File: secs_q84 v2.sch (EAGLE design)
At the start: 107 parts, among them IC1 MAX203ECWP, IC2 REF3440TIDBVR, IC3 ADP151AUJZ-3.3-R7, IC4 PIC18F47Q84-I_PT, IC5 MCZ33996EK, IC6 74HC125D, IC7 TIC12400DCPR

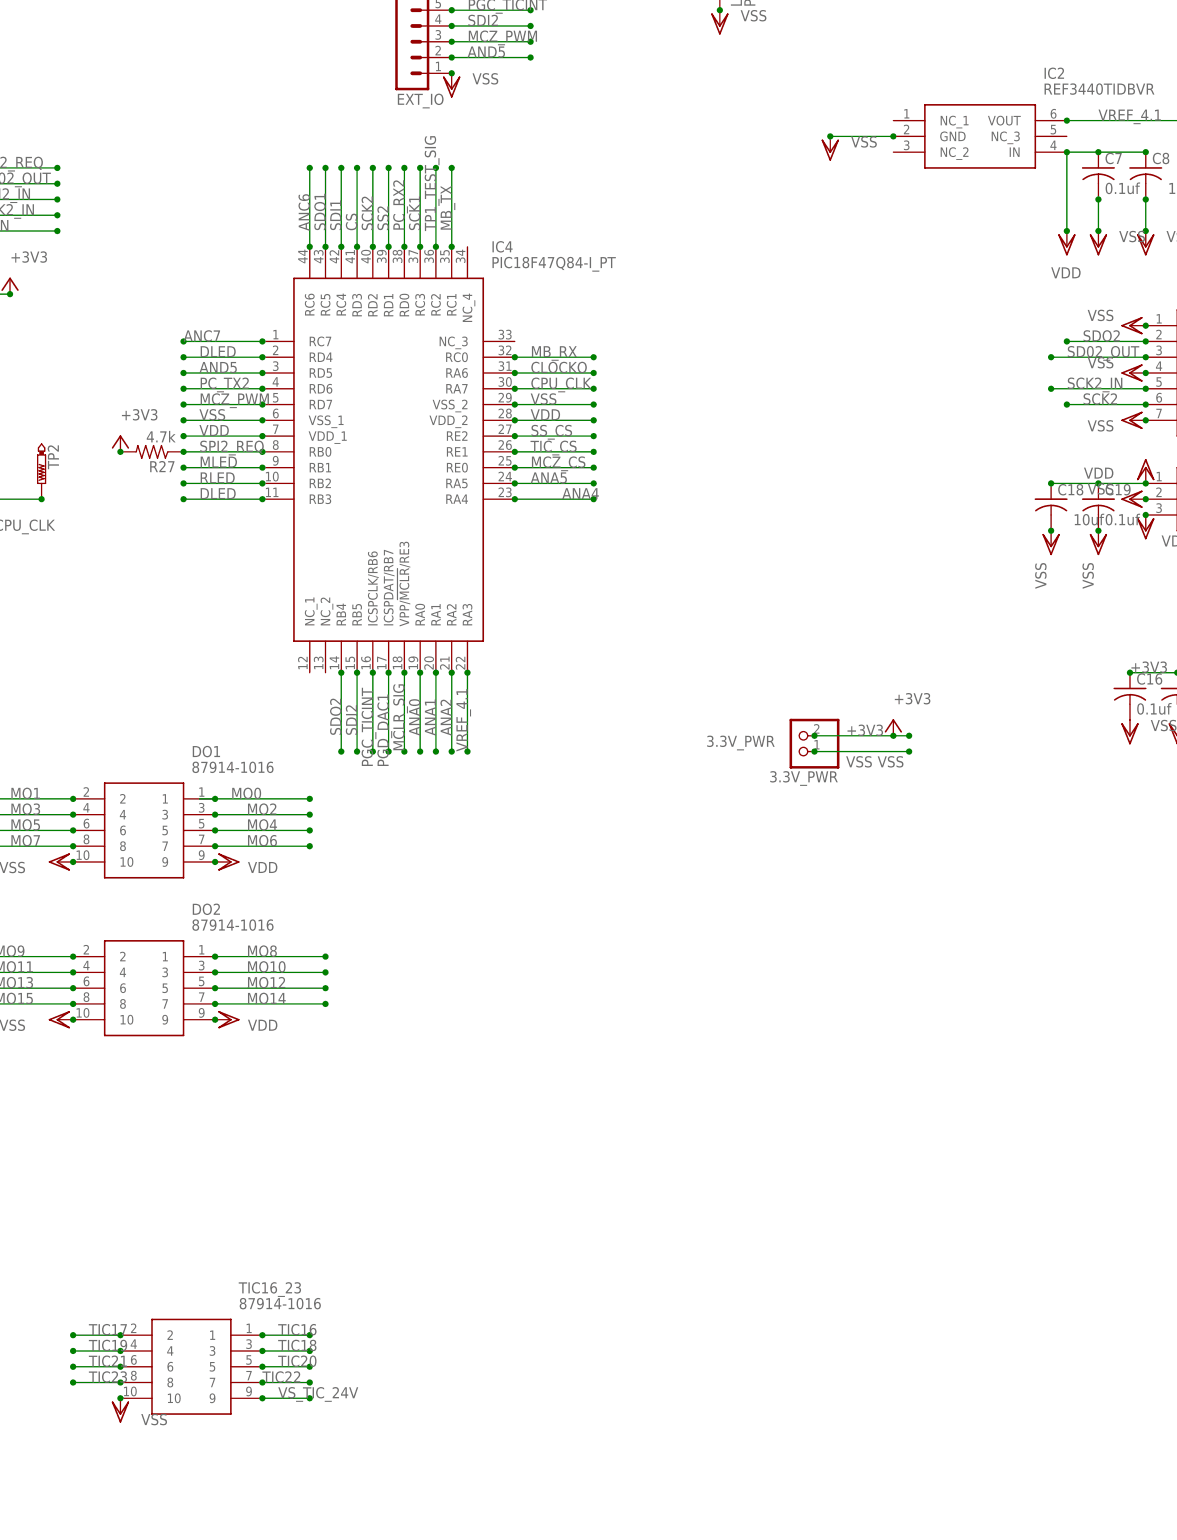
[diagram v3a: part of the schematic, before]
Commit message: up uuuppp#	modified:   secs_q84 v2.b#5
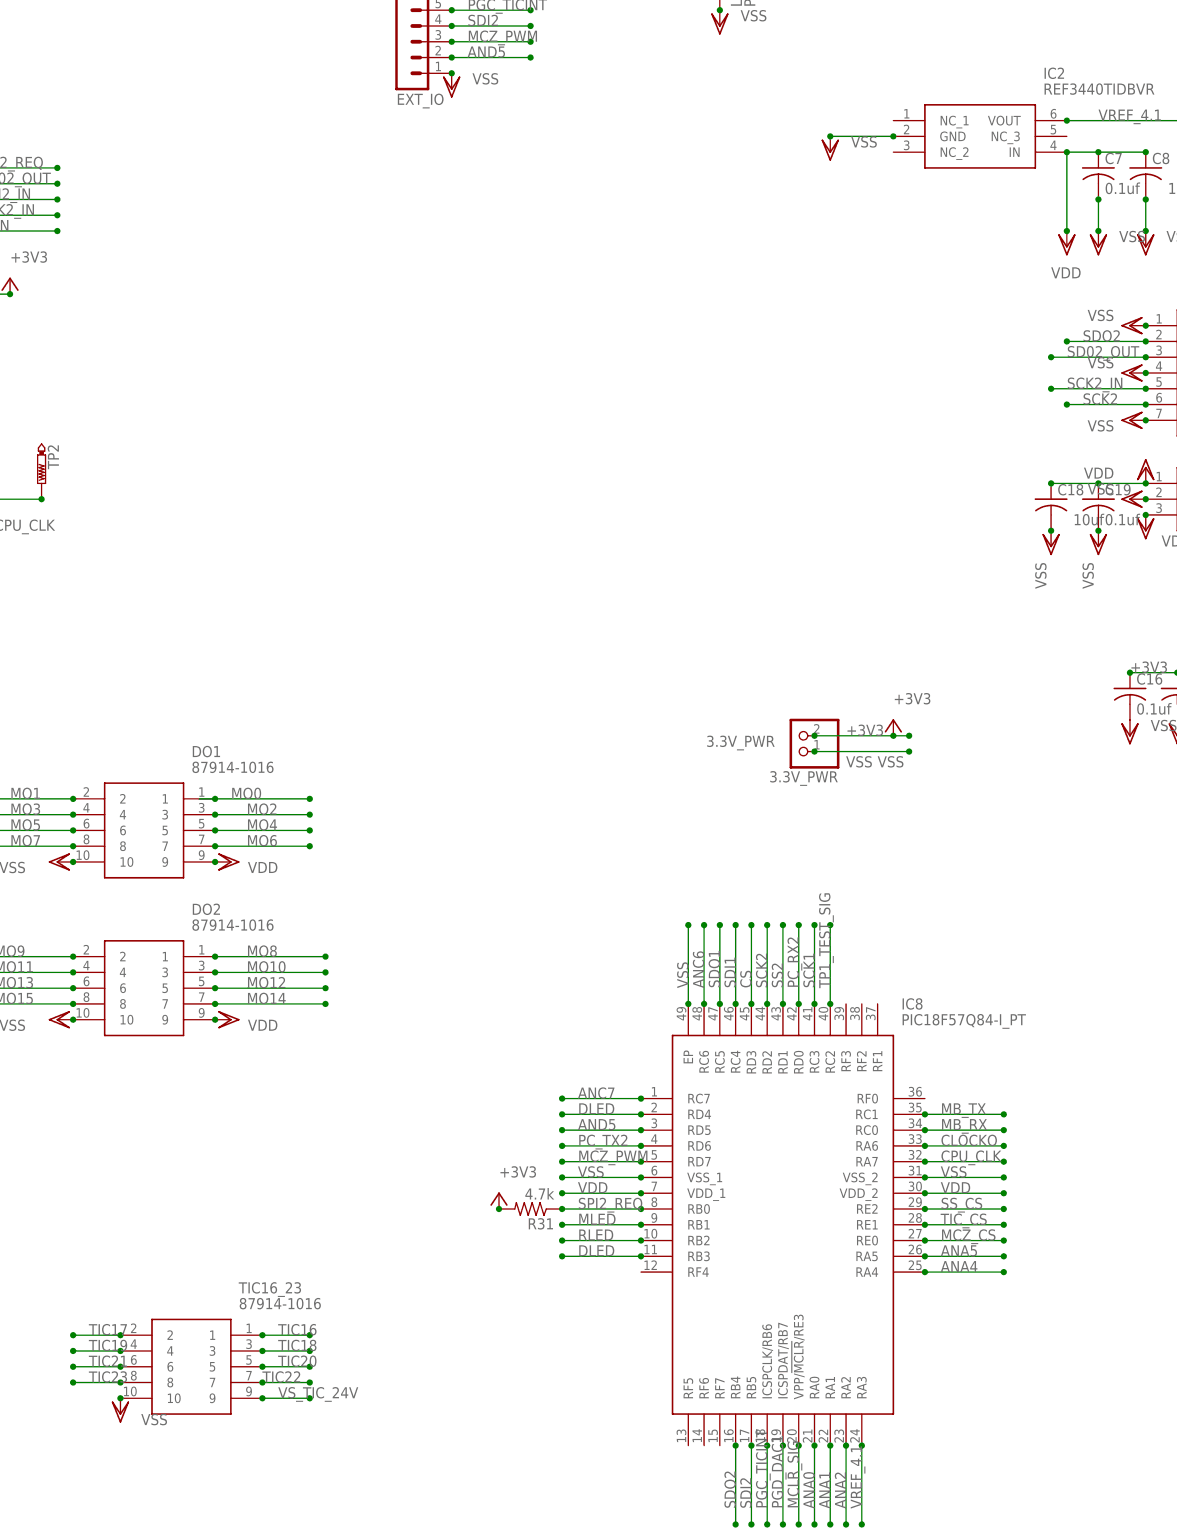
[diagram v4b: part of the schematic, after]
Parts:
- removed IC4: PIC18F47Q84-I_PT, PIC18F47Q84-I_PT:PIC18F47Q84-I_PT
- removed R27: 4.7k, rcl:R-US_R0805
- added IC8: PIC18F57Q84-I_PT, PIC18F57Q84-I_PT:PIC18F57Q84-I_PT
- added R31: 4.7k, rcl:R-US_R0805
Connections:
- net +3V3: now also R31.2; no longer R27.2
- net ANA0: now also IC8.RA0; no longer IC4.RA0
- net ANA1: now also IC8.RA1; no longer IC4.RA1
- net ANA2: now also IC8.RA2; no longer IC4.RA2
- net ANA4: now also IC8.RA4; no longer IC4.RA4
- net ANA5: now also IC8.RA5; no longer IC4.RA5
- net ANC6: now also IC8.RC6; no longer IC4.RC6
- net ANC7: now also IC8.RC7; no longer IC4.RC7
- net AND5: now also IC8.RD5; no longer IC4.RD5
- net CLOCKO: now also IC8.RA6; no longer IC4.RA6
- net CPU_CLK: now also IC8.RA7; no longer IC4.RA7
- net CS: now also IC8.RD3; no longer IC4.RD3
- net DLED: now also IC8.RB3, IC8.RD4; no longer IC4.RB3, IC4.RD4
- net MB_RX: now also IC8.RC0; no longer IC4.RC0
- net MB_TX: now also IC8.RC1; no longer IC4.RC1
- net MCLR_SIG: now also IC8.VPP/!MCLR!/RE3; no longer IC4.VPP/!MCLR!/RE3
- net MCZ_CS: now also IC8.RE0; no longer IC4.RE0
- net MCZ_PWM: now also IC8.RD7; no longer IC4.RD7
- net MLED: now also IC8.RB1; no longer IC4.RB1
- net PC_RX2: now also IC8.RD0; no longer IC4.RD0
- net PC_TX2: now also IC8.RD6; no longer IC4.RD6
- net PGC_TICINT: now also IC8.ICSPCLK/RB6; no longer IC4.ICSPCLK/RB6
- net PGD_DAC1: now also IC8.ICSPDAT/RB7; no longer IC4.ICSPDAT/RB7
- net RLED: now also IC8.RB2; no longer IC4.RB2
- net SCK1: now also IC8.RC3; no longer IC4.RC3
- net SCK2: now also IC8.RD2; no longer IC4.RD2
- net SDI1: now also IC8.RC4; no longer IC4.RC4
- net SDI2: now also IC8.RB5; no longer IC4.RB5
- net SDO1: now also IC8.RC5; no longer IC4.RC5
- net SDO2: now also IC8.RB4; no longer IC4.RB4
- net SPI2_REQ: now also IC8.RB0, R31.1; no longer IC4.RB0, R27.1
- net SS2: now also IC8.RD1; no longer IC4.RD1
- net SS_CS: now also IC8.RE2; no longer IC4.RE2
- net TIC_CS: now also IC8.RE1; no longer IC4.RE1
- net TP1_TEST_SIG: now also IC8.RC2; no longer IC4.RC2
- net VDD: now also IC8.VDD_1, IC8.VDD_2; no longer IC4.VDD_1, IC4.VDD_2
- net VREF_4.1: now also IC8.RA3; no longer IC4.RA3
- net VSS: now also IC8.EP, IC8.VSS_1, IC8.VSS_2; no longer IC4.VSS_1, IC4.VSS_2
